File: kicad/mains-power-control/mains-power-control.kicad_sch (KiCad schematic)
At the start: 25 parts, among them J1 Conn_01x04_Socket, J2 Conn_01x06_Pin, J3 Conn_01x03_Pin, J4 Conn_01x03_Pin, J5 Conn_01x04_Pin, J9 Conn_01x03_Pin, Q1 ZVN4206AV, U1 BP, U2 SeeeduinoXIAO, U3 MOC3020M, U5 H11AA1

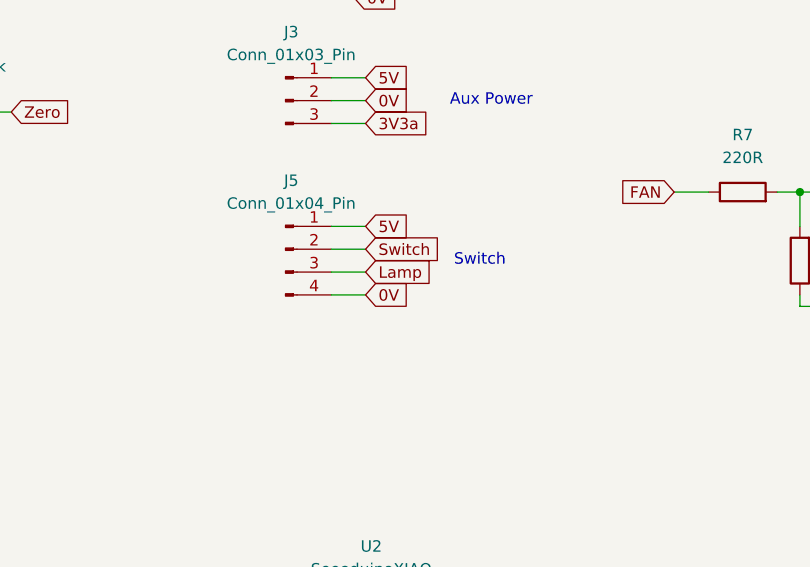
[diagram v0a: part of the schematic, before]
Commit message: PCB v 1.1
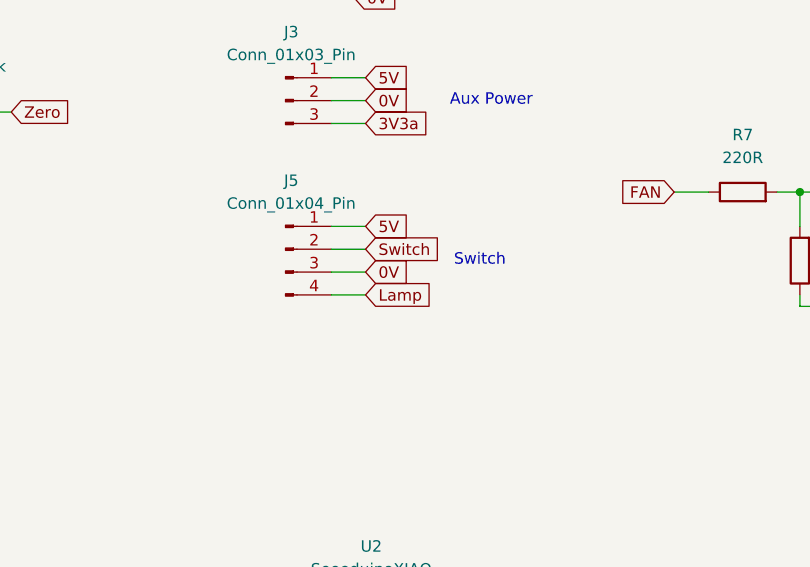
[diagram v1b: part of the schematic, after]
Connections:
- net 0V: now also J5.3 (Pin_3); no longer J5.4 (Pin_4)
- net Lamp: now also J5.4 (Pin_4); no longer J5.3 (Pin_3)
